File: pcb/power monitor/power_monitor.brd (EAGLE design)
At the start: 22.9 x 30.5 mm, 17 parts, among them IC1 MAX4105ESA, IC2 MAX4105ESA, IC3 MAX4105ESA

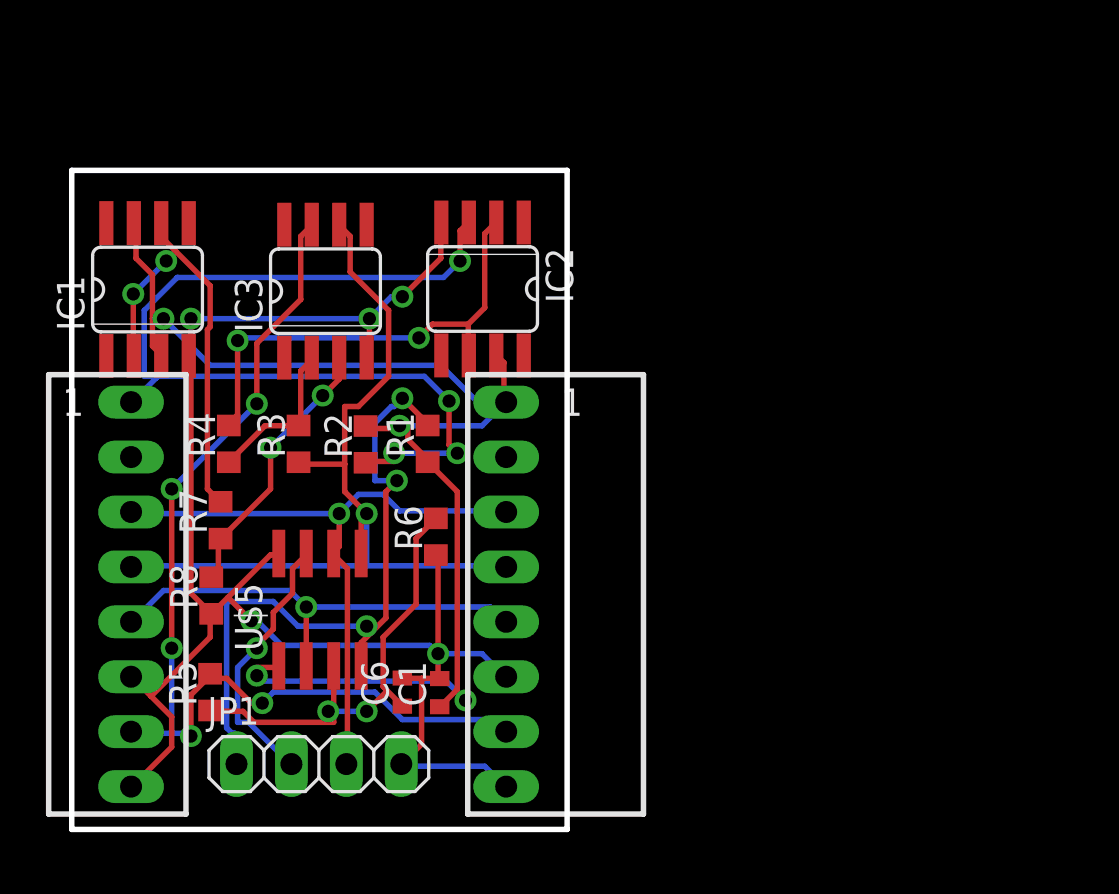
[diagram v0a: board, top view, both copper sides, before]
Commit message: Signed-off-by: timcronin <tmpcronin@gmail.com>
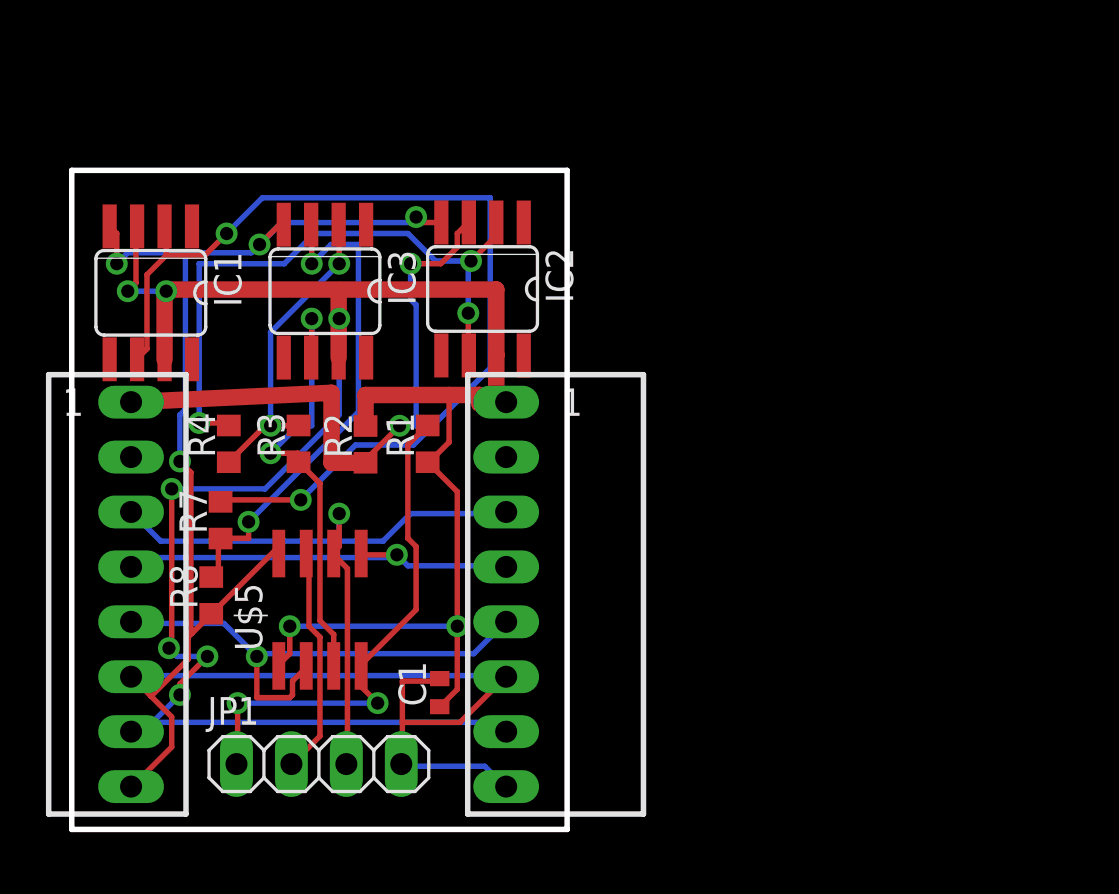
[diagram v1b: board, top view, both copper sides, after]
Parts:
- removed C6: 100 nF, rcl:C0402
- removed R5, R6: 500K, rcl:R0603
- moved IC1 0.22 mm to (3.61, 24.8), turned to 180 degrees
- turned IC3 to 180 degrees
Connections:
- removed net N$5: C6.1, R5.1, R6.2, U$5.3
- new net N$2: IC3.6, R3.1, U$5.3
- net DAT: no longer IC3.6, R3.1
- net GND: no longer C6.2, R6.1
- net V+: no longer R5.2
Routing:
- net N$4: track 19.8 -> 45.8 mm
- net N$5: track 22.0 -> 0.00 mm, vias 2 -> 0
- net N$2: track 0.00 -> 21.0 mm, vias 0 -> 2
- net DAT: track 39.9 -> 19.6 mm
- net N$11: track 44.0 -> 28.6 mm, vias 4 -> 2
- net N$9: track 12.6 -> 23.3 mm
- net GND: track 77.9 -> 87.7 mm, vias 5 -> 4
- net N$1: track 31.6 -> 24.1 mm, vias 3 -> 2
- net N$3: track 21.8 -> 29.1 mm, vias 2 -> 3
- net N$7: track 7.32 -> 14.6 mm, vias 0 -> 2
- net IRQ: track 21.3 -> 23.9 mm
- net V+: track 47.6 -> 49.8 mm
- net VCCINT: track 61.4 -> 63.3 mm
- net N$8: track 12.4 -> 10.6 mm, vias 1 -> 0
- net CLK: track 30.1 -> 31.7 mm

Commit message: Signed-off-by: timcronin <tmpcronin@gmail.com>
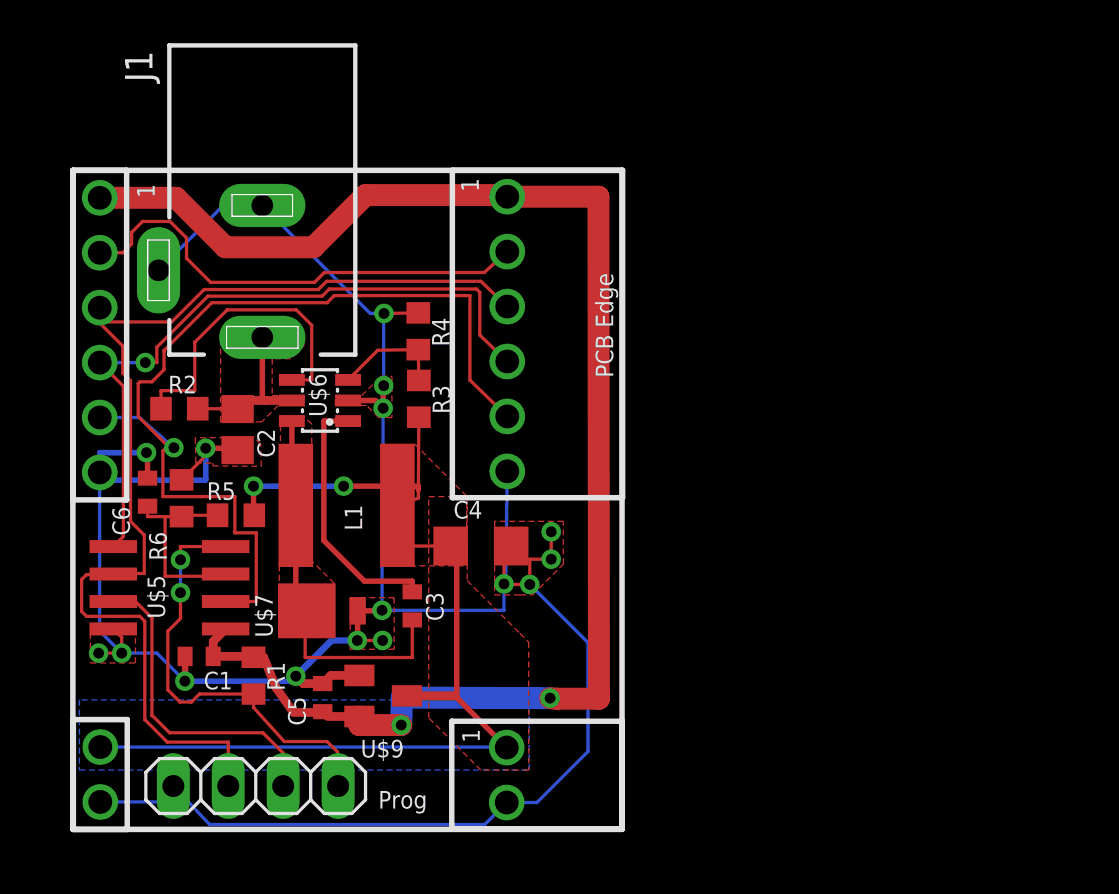
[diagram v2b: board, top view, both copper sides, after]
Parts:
- removed IC1, IC2, IC3: MAX4105ESA, maxim:SO08
- removed R7: 1k, rcl:R0603
- removed R8: 69.8k, rcl:R0603
- added C2: 10 uF, rcl:C0805
- added C3: 10 nF, rcl:C0402
- added C4: 22 uF, rcl:C1206
- added C5: 22 uF, rcl:C0402
- added C6: 100 nF, rcl:C0402
- added J1: (no value), con-jack:DCJ0303
- added R5, R6: 500K, rcl:R0603
- added U$1: MOMO-EDGE-SMALL-M, components:MOMO-EDGE-SMALL-6M
- added U$2: MOMO-EDGE-SMALL-F, components:MOMO-EDGE-SMALL-6F
- added U$3: MOMO-EDGE-POWER-M, components:MOMO-EDGE-SMALL-2M
- added U$4: MOMO-EDGE-POWER-F, components:MOMO-EDGE-SMALL-2F
- added U$8: 4.7 uH, components:NR6028-INDUCTOR
- added U$9: MCP1702, components:SOT23
- R2: value 2 -> 100K
- R3: value 69.8k -> 50K 1%
- R4: value 1k -> 13K 1%
- U$6: value MOMO-EDGE-8F -> XRP7659; device components:MOMO-EDGE-8F -> components:SOT23-6L
- U$7: value MOMO-EDGE-8M -> DIODE_SS2P3; device components:MOMO-EDGE-8M -> components:DIODE_SS2P3
- moved R1 13.4 mm to (8.36, 7.11), turned to 270 degrees
- moved U$6 13.4 mm to (11.4, 19.8), turned to 90 degrees
- moved C1 11.3 mm to (5.84, 8.00), turned to 180 degrees
- moved R4 10.2 mm to (16.0, 23.0), turned to 270 degrees
- moved R2 8.77 mm to (4.93, 19.5), turned to 180 degrees
- moved U$7 8.14 mm to (10.8, 10.1)
- moved U$5 7.03 mm to (4.47, 11.2), turned to 90 degrees
- moved R3 5.94 mm to (16.0, 19.9), turned to 270 degrees
- moved JP1 3.09 mm to (8.46, 2.01), turned to 180 degrees
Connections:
- removed net N$11: IC2.3, R2.1, U$7.V28
- removed net N$7: IC3.2, R3.2, R4.1
- removed net N$9: IC3.3, R7.1, R8.2
- new net +12V: C2.1, J1.1, R2.1, U$6.5
- new net N$5: C6.1, R5.1, R6.2, U$5.3
- new net N$6: R3.1, R4.2, U$6.3
- new net NC: U$1.2, U$2.2
- net CLK: now also U$1.3, U$2.3; no longer U$6.CLK, U$7.CLK
- net DAT: now also U$1.4, U$2.4; no longer U$6.DAT, U$7.DAT
- net GND: now also C2.2, C4.2, C5.2, C6.2, J1.2, J1.3, R4.1, R6.1, U$1.6, U$2.6, U$3.2, U$4.2, U$6.2, U$7.AN, U$9.1; no longer IC1.4, IC2.4, IC3.4, R8.1, U$6.GND, U$6.PGND, U$7.GND, U$7.PGND
- net IRQ: now also U$1.5, U$2.5; no longer U$6.ARLM, U$7.ALRM
- net N$2: now also C3.2, U$6.6, U$7.CATH, U$8.1; no longer IC3.6, R3.1, U$5.3
- net N$3: now also R2.2, U$6.4; no longer IC2.2, IC2.6, R4.2
- net N$4: now also C3.1, U$6.1; no longer IC1.2, IC1.6, R7.2
- net V+: now also C4.1, R3.2, R5.2, U$3.1, U$4.1, U$8.2, U$9.3; no longer IC3.7, U$6.V4., U$7.V4
- net VCCINT: now also C5.1, U$1.1, U$2.1, U$9.2; no longer IC1.3, IC1.7, IC2.7, R2.2, U$6.V28
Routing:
- net GND: track 87.7 -> 129.5 mm, vias 4 -> 16
- net N$4: track 45.8 -> 12.0 mm, vias 2 -> 0
- net N$11: track 28.6 -> 0.00 mm, vias 2 -> 0
- net N$9: track 23.3 -> 0.00 mm, vias 2 -> 0
- net NC: track 0.00 -> 22.0 mm
- net IRQ: track 23.9 -> 44.9 mm
- net CLK: track 31.7 -> 51.7 mm, vias 1 -> 0
- net N$3: track 29.1 -> 14.4 mm, vias 3 -> 0
- net N$7: track 14.6 -> 0.00 mm, vias 2 -> 0
- net DAT: track 19.6 -> 32.4 mm
- net N$5: track 0.00 -> 9.44 mm
- net +12V: track 0.00 -> 7.81 mm
- net VCCINT: track 63.3 -> 70.9 mm, vias 4 -> 2
- net N$6: track 0.00 -> 5.24 mm
- net N$8: track 10.6 -> 14.9 mm
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- added copper zone on layer 1, net +12V
- added copper zone on layer 1, net GND
- added copper zone on layer 16, net GND
- added copper zone on layer 1, net N$2
- added copper zone on layer 1, net V+
- added copper zone on layer 16, net V+
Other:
- board size 22.9 x 30.5 mm -> 7 x 7.1 mm
- board text added: "L1"
- board text added: "Prog"

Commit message: Signed-off-by: timcronin <tmpcronin@gmail.com>
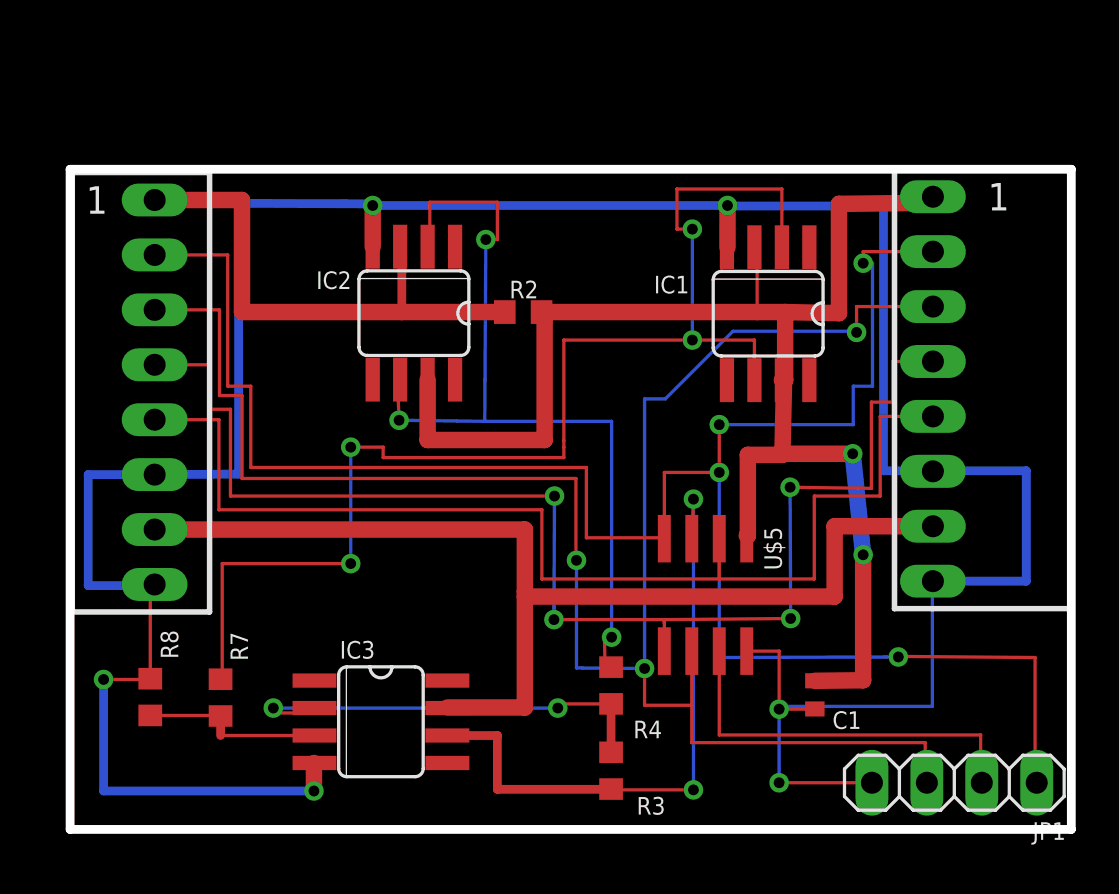
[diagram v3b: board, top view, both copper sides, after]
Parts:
- removed C2: 10 uF, rcl:C0805
- removed C3: 10 nF, rcl:C0402
- removed C4: 22 uF, rcl:C1206
- removed C5: 22 uF, rcl:C0402
- removed C6: 100 nF, rcl:C0402
- removed J1: (no value), con-jack:DCJ0303
- removed R1: 10K, rcl:R0603
- removed R5, R6: 500K, rcl:R0603
- removed U$1: MOMO-EDGE-SMALL-M, components:MOMO-EDGE-SMALL-6M
- removed U$2: MOMO-EDGE-SMALL-F, components:MOMO-EDGE-SMALL-6F
- removed U$3: MOMO-EDGE-POWER-M, components:MOMO-EDGE-SMALL-2M
- removed U$4: MOMO-EDGE-POWER-F, components:MOMO-EDGE-SMALL-2F
- removed U$8: 4.7 uH, components:NR6028-INDUCTOR
- removed U$9: MCP1702, components:SOT23
- added IC1, IC2, IC3: MAX4105ESA, maxim:SO08
- added R7: 1k, rcl:R0603
- added R8: 69.8k, rcl:R0603
- R2: value 100K -> 2
- R3: value 50K 1% -> 69.8k
- R4: value 13K 1% -> 1k
- U$6: value XRP7659 -> MOMO-EDGE-8F; device components:SOT23-6L -> components:MOMO-EDGE-8F
- U$7: value DIODE_SS2P3 -> MOMO-EDGE-8M; device components:DIODE_SS2P3 -> components:MOMO-EDGE-8M
- moved JP1 32.3 mm to (40.8, 2.16)
- moved C1 28.5 mm to (34.3, 6.22), turned to 270 degrees
- moved U$6 28.4 mm to (39.8, 19.1), turned to 0 degrees
- moved U$5 24.8 mm to (29.3, 10.8), turned to 180 degrees
- moved R3 19.4 mm to (24.9, 2.72), turned to 90 degrees
- moved R4 18.7 mm to (24.9, 6.65), turned to 90 degrees
- moved R2 16.5 mm to (20.8, 23.9), turned to 0 degrees
- moved U$7 11.3 mm to (3.78, 18.9)
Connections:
- removed net +12V: C2.1, J1.1, R2.1, U$6.5
- removed net N$5: C6.1, R5.1, R6.2, U$5.3
- removed net N$6: R3.1, R4.2, U$6.3
- removed net NC: U$1.2, U$2.2
- new net N$11: IC2.3, R2.1, U$7.V28
- new net N$7: IC3.2, R3.2, R4.1
- new net N$9: IC3.3, R7.1, R8.2
- net CLK: now also U$6.CLK, U$7.CLK; no longer U$1.3, U$2.3
- net DAT: now also U$6.DAT, U$7.DAT; no longer U$1.4, U$2.4
- net GND: now also IC1.4, IC2.4, IC3.4, R8.1, U$6.GND, U$6.PGND, U$7.GND, U$7.PGND; no longer C2.2, C4.2, C5.2, C6.2, J1.2, J1.3, R4.1, R6.1, U$1.6, U$2.6, U$3.2, U$4.2, U$6.2, U$7.AN, U$9.1
- net IRQ: now also U$6.ARLM, U$7.ALRM; no longer U$1.5, U$2.5
- net N$1: now also U$6.NV, U$7.NC; no longer R1.2
- net N$2: now also IC3.6, R3.1, U$5.3; no longer C3.2, U$6.6, U$7.CATH, U$8.1
- net N$3: now also IC2.2, IC2.6, R4.2; no longer R2.2, U$6.4
- net N$4: now also IC1.2, IC1.6, R7.2; no longer C3.1, U$6.1
- net V+: now also IC3.7, U$6.V4., U$7.V4; no longer C4.1, R3.2, R5.2, U$3.1, U$4.1, U$8.2, U$9.3
- net VCCINT: now also IC1.3, IC1.7, IC2.7, R2.2, U$6.V28; no longer C5.1, R1.1, U$1.1, U$2.1, U$9.2
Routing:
- net N$1: track 20.5 -> 92.3 mm, vias 2 -> 4
- net N$4: track 12.0 -> 58.4 mm, vias 0 -> 4
- net CLK: track 51.7 -> 88.4 mm, vias 0 -> 3
- net DAT: track 32.4 -> 61.2 mm, vias 1 -> 4
- net N$3: track 14.4 -> 39.7 mm, vias 0 -> 3
- net N$11: track 0.00 -> 24.5 mm
- net NC: track 22.0 -> 0.00 mm
- net N$7: track 0.00 -> 20.3 mm, vias 0 -> 2
- net N$2: track 18.1 -> 29.2 mm, vias 0 -> 2
- net GND: track 129.5 -> 139.4 mm, vias 16 -> 6
- net N$5: track 9.44 -> 0.00 mm
- net N$9: track 0.00 -> 8.52 mm
- net IRQ: track 44.9 -> 52.7 mm, vias 1 -> 0
- net +12V: track 7.81 -> 0.00 mm
- net N$6: track 5.24 -> 0.00 mm
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- added copper zone on layer 16, net N$5
- removed copper zone on layer 1, net +12V
- removed copper zone on layer 1, net GND
- removed copper zone on layer 16, net GND
- removed copper zone on layer 1, net N$2
- removed copper zone on layer 1, net V+
- removed copper zone on layer 16, net V+
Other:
- board size 7 x 7.1 mm -> 46.3 x 30.5 mm
- board text removed: "L1"
- board text removed: "Prog"
